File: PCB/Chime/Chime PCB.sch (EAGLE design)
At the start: 36 parts, among them J1_SPI 1725698, J2_I2C 1725672, J4_A1 1725669, J5_A0 1725669, U1 MS5803-02BA, X4 BQ24074

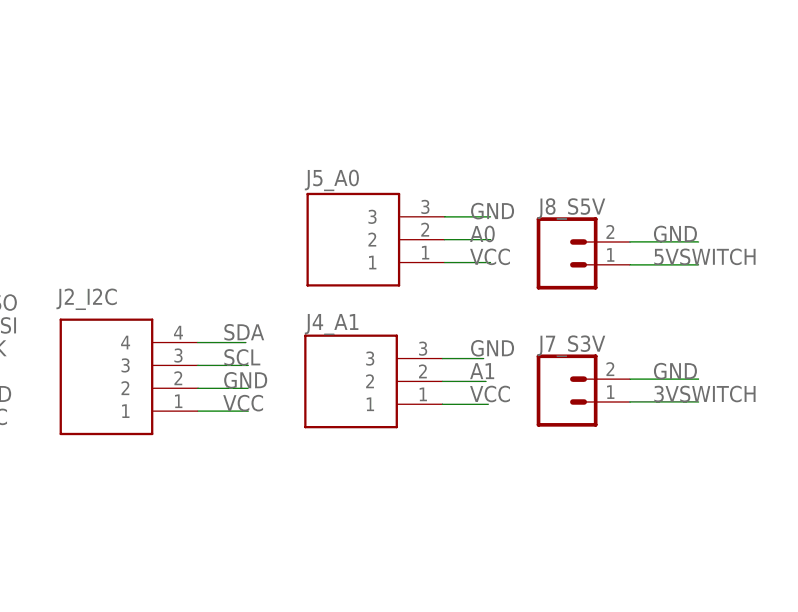
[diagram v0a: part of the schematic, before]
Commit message: Add files via upload
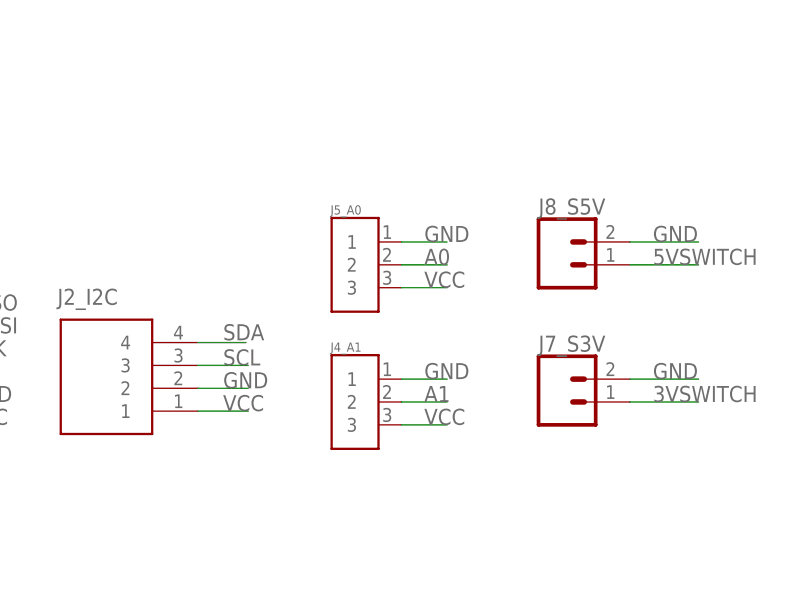
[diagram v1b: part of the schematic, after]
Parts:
- J4_A1, J5_A0: value 1725669 -> 282834-3; device 1725669:1725669 -> Fixed Terminal Blocks 3P:282834-3
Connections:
- net GND: now also J4_A1.1, J5_A0.1; no longer J4_A1.3, J5_A0.3
- net VCC: now also J4_A1.3, J5_A0.3; no longer J4_A1.1, J5_A0.1
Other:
- moved on the sheet: J4_A1, J5_A0
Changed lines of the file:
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@@
 <part name="J2_I2C" library="1725672" deviceset="1725672" device=""/>
 <part name="J1_SPI" library="1725698" deviceset="1725698" device=""/>
-<part name="J4_A1" library="1725669" deviceset="1725669" device=""/>
-<part name="J5_A0" library="1725669" deviceset="1725669" device=""/>
 <part name="U$17" library="microbuilder" deviceset="MOUNTINGHOLE" device="2.5"/>
 <part name="U$19" library="microbuilder" deviceset="MOUNTINGHOLE" device="2.5"/>
@@
 <part name="J8_S5V" library="SparkFun-Connectors" deviceset="CONN_02" device=""/>
 <part name="SJ1" library="SparkFun-Jumpers" library_urn="urn:adsk.eagle:library:528" deviceset="JUMPER-SMT_3_1-NC_TRACE" device="_SILK" package3d_urn="urn:adsk.eagle:package:39288/1"/>
+<part name="J4_A1" library="Fixed Terminal Blocks 3P" deviceset="282834-3" device=""/>
+<part name="J5_A0" library="Fixed Terminal Blocks 3P" deviceset="282834-3" device=""/>
 </parts>
 <sheets>
@@
 <attribute name="NAME" x="273.812" y="78.486" size="1.778" layer="95" rot="R180" align="center-left"/>
 </instance>
-<instance part="J4_A1" gate="G$1" x="339.852" y="63.246" smashed="yes" rot="R180">
-<attribute name="NAME" x="330.708" y="72.39" size="1.778" layer="95" rot="R180" align="center-left"/>
-</instance>
-<instance part="J5_A0" gate="G$1" x="340.106" y="78.994" smashed="yes" rot="R180">
-<attribute name="NAME" x="330.708" y="88.392" size="1.778" layer="95" rot="R180" align="center-left"/>
-</instance>
 <instance part="U$17" gate="G$1" x="271.018" y="44.45" smashed="yes"/>
 <instance part="U$19" gate="G$1" x="271.272" y="38.354" smashed="yes"/>
@@
 <instance part="SJ1" gate="G$1" x="127" y="127" smashed="yes" grouprefs="MS580302BA">
 <attribute name="NAME" x="129.286" y="126.873" size="1.778" layer="95"/>
+</instance>
+<instance part="J4_A1" gate="G$1" x="330.2" y="63.5" smashed="yes">
+<attribute name="NAME" x="327.40435" y="69.091309375" size="1.0166" layer="95"/>
+</instance>
+<instance part="J5_A0" gate="G$1" x="330.2" y="78.74" smashed="yes">
+<attribute name="NAME" x="327.40435" y="84.331309375" size="1.0166" layer="95"/>
 </instance>
 </instances>
@@
 </segment>
 <segment>
-<pinref part="J4_A1" gate="G$1" pin="3"/>
-<wire x1="339.852" y1="68.326" x2="344.424" y2="68.326" width="0.1524" layer="91"/>
-<label x="342.9" y="68.58" size="1.778" layer="95"/>
-</segment>
-<segment>
-<pinref part="J5_A0" gate="G$1" pin="3"/>
-<wire x1="340.106" y1="84.074" x2="345.186" y2="84.074" width="0.1524" layer="91"/>
-<label x="342.9" y="83.82" size="1.778" layer="95"/>
-</segment>
-<segment>
 <pinref part="J6_TSL2591" gate="JP1" pin="3"/>
 <wire x1="279.4" y1="93.98" x2="287.02" y2="93.98" width="0.1524" layer="91"/>
@@
 <pinref part="GND10" gate="1" pin="GND"/>
 <wire x1="116.84" y1="45.72" x2="116.84" y2="48.26" width="0.1524" layer="91"/>
+</segment>
+<segment>
+<pinref part="J4_A1" gate="G$1" pin="1"/>
+<wire x1="335.28" y1="66.04" x2="340.36" y2="66.04" width="0.1524" layer="91"/>
+<label x="337.82" y="66.04" size="1.778" layer="95"/>
+</segment>
+<segment>
+<pinref part="J5_A0" gate="G$1" pin="1"/>
+<wire x1="335.28" y1="81.28" x2="340.36" y2="81.28" width="0.1524" layer="91"/>
+<label x="337.82" y="81.28" size="1.778" layer="95"/>
 </segment>
 </net>
@@
 </segment>
 <segment>
-<pinref part="J4_A1" gate="G$1" pin="1"/>
-<wire x1="339.852" y1="63.246" x2="344.932" y2="63.246" width="0.1524" layer="91"/>
-<label x="342.9" y="63.5" size="1.778" layer="95"/>
-</segment>
-<segment>
-<pinref part="J5_A0" gate="G$1" pin="1"/>
-<wire x1="340.106" y1="78.994" x2="345.186" y2="78.994" width="0.1524" layer="91"/>
-<label x="342.9" y="78.74" size="1.778" layer="95"/>
-</segment>
-<segment>
 <pinref part="J6_TSL2591" gate="JP1" pin="2"/>
 <wire x1="279.4" y1="91.44" x2="287.02" y2="91.44" width="0.1524" layer="91"/>
 <label x="281.94" y="91.44" size="1.778" layer="95"/>
 </segment>
+<segment>
+<pinref part="J4_A1" gate="G$1" pin="3"/>
+<wire x1="335.28" y1="60.96" x2="340.36" y2="60.96" width="0.1524" layer="91"/>
+<label x="337.82" y="60.96" size="1.778" layer="95"/>
+</segment>
+<segment>
+<pinref part="J5_A0" gate="G$1" pin="3"/>
+<wire x1="335.28" y1="76.2" x2="340.36" y2="76.2" width="0.1524" layer="91"/>
+<label x="337.82" y="76.2" size="1.778" layer="95"/>
+</segment>
 </net>
 <net name="A1" class="0">
@@
 <segment>
 <pinref part="J4_A1" gate="G$1" pin="2"/>
-<wire x1="339.852" y1="65.786" x2="344.678" y2="65.786" width="0.1524" layer="91"/>
-<label x="342.9" y="66.04" size="1.778" layer="95"/>
+<wire x1="335.28" y1="63.5" x2="340.36" y2="63.5" width="0.1524" layer="91"/>
+<label x="337.82" y="63.5" size="1.778" layer="95"/>
 </segment>
 </net>
@@
 <segment>
 <pinref part="J5_A0" gate="G$1" pin="2"/>
-<wire x1="340.106" y1="81.534" x2="345.186" y2="81.534" width="0.1524" layer="91"/>
-<label x="342.9" y="81.28" size="1.778" layer="95"/>
-</segment>
-</net>
+<wire x1="335.28" y1="78.74" x2="340.36" y2="78.74" width="0.1524" layer="91"/>
+<label x="337.82" y="78.74" size="1.778" layer="95"/>
+</segment>
+</net>
